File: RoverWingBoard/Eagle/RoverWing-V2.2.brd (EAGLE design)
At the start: 81.3 x 81.3 mm, 91 parts, among them J1 XT30UPB-M, J10 HEADER-3X04, J11 HEADER-3X06ANGLE, J12 HEADER-2X16, J13 HEADER-2X12, J14 DF13-4P-1.25DSA, J15 DF13-6P-1.25DSA, J16 HEADER-SH-4P, J2 HEADER-VH, J3 HEADER-VH, J4 HEADER-PH-4P, J5 HEADER-PH-4P, J6 HEADER-PH-4P, J7 HEADER-PH-4P, J8 HEADER-PH-4P, J9 HEADER-PH-3P, SW1 SW-TACTILE-4.5X4.5_SMD, U1 ATSAMD21G, U2 TPS54531, U3 PMIC-AZ1117EH-3.3, U4 ICM-42605, U5 DRV8871, U6 DRV8871, U7 74AHCT1G125DBV

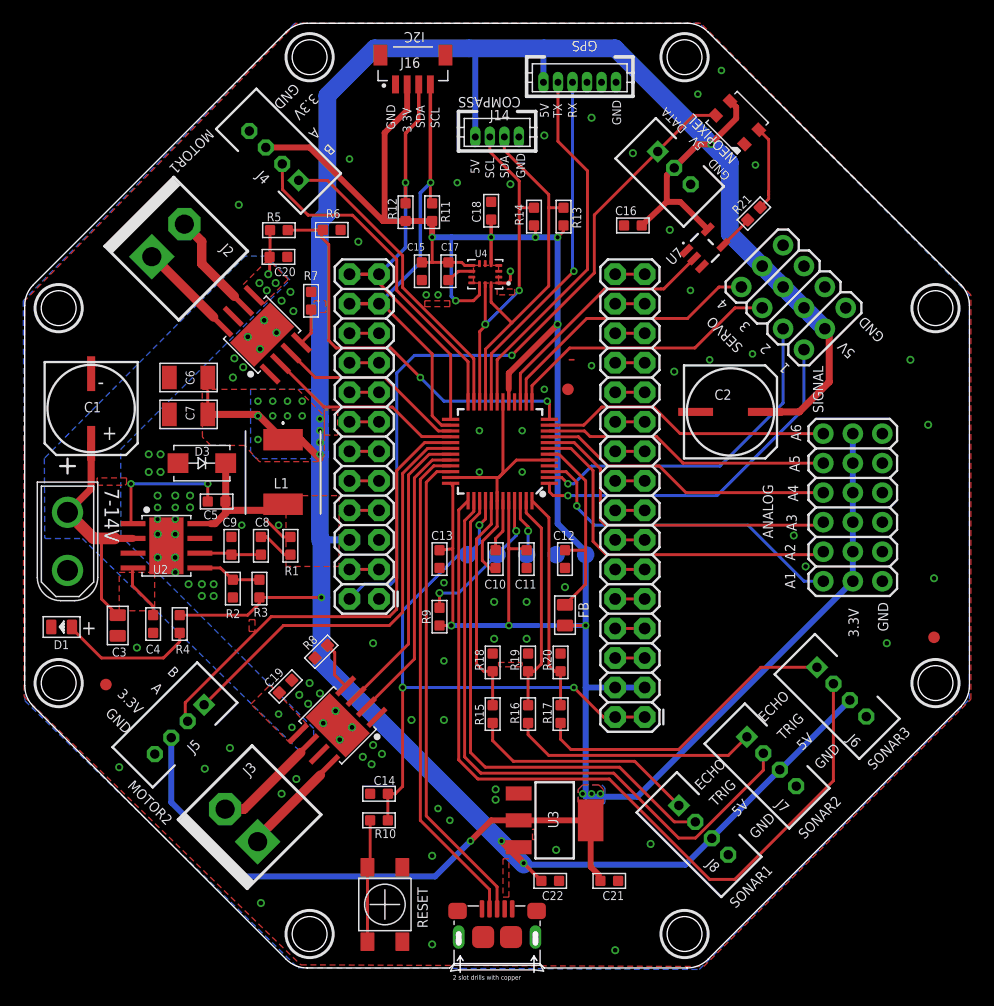
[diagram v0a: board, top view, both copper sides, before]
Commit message: acknowledgment of copperforge.cc  theme
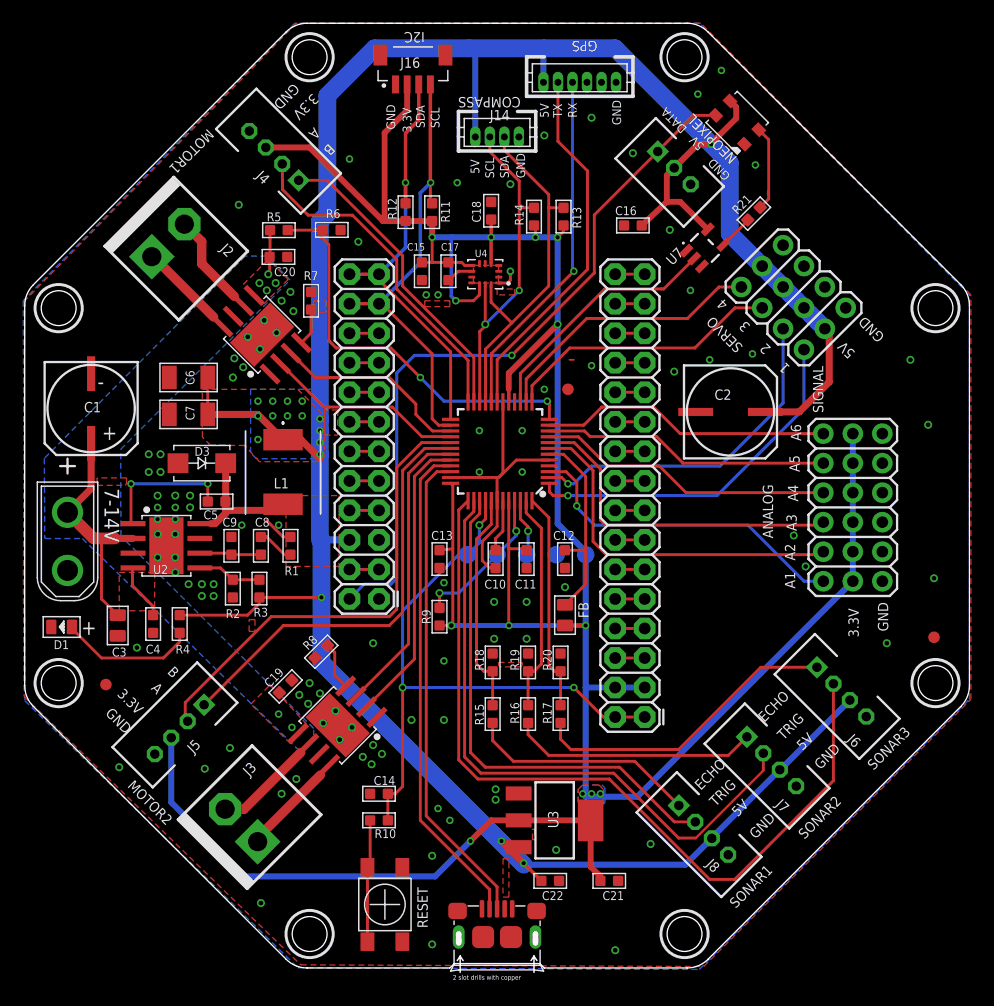
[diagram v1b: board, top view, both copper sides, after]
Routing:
- net 3.3V: track 260.9 -> 261.4 mm
- net MOTOR1A: track 16.5 -> 17.0 mm
